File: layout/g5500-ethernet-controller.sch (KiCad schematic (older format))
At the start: 71 parts, among them IC1 MAX-M8Q, J1 CONN_01x03, J10 CONN_01x03, J11 CONN_01x02, J2 CONN_01x03, J3 MICROUSB, J4 CONN_01x02, J5 CONN_01x03, J6 CONN_01x03, J7 CONN_01x02, J8 CONN_01x02, J9 CONN_01x03, K1 G5LE-1, K2 G5LE-1, K3 G5LE-1, K4 G5LE-1, P1 COAX, Q1 BC817W, Q2 BC817W, Q3 BC817W, Q4 BC817W, U1 NUCLEO144-F429ZI, U2 LD3985G33R_TSOT23

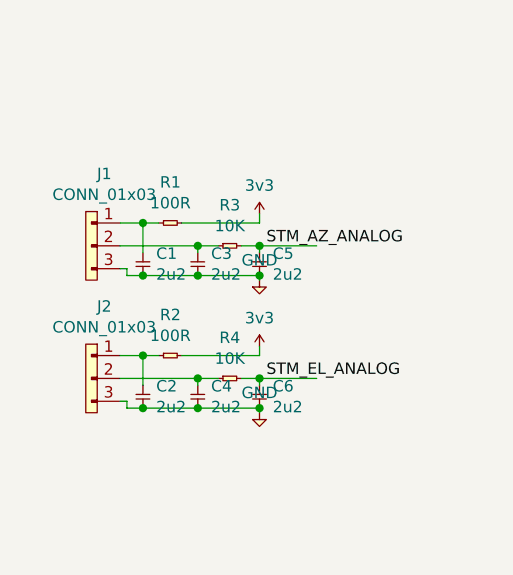
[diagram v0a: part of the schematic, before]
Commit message: layout: Finish and send off v1.
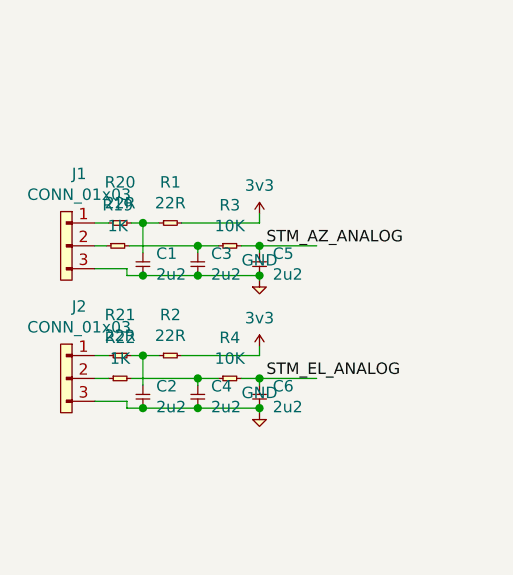
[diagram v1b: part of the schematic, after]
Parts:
- added R19, R22: 1K, agg:0603, symbol agg-kicad:R
- added R20, R21: 22R, agg:0603, symbol agg-kicad:R
- C13: footprint Capacitor_SMD:C_0603_1608Metric -> agg:0603
- R1, R2: value 100R -> 22R
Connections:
- wire segments 263 -> 267
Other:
- moved on the sheet: J1, J2
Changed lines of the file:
@@
 L agg-kicad:CONN_01x03 J2
 U 1 1 5A89F92A
-P 1680 7890
-F 0 "J2" H 1711 8105 50  0000 C CNN
-F 1 "CONN_01x03" H 1711 8014 50  0000 C CNN
-F 2 "Connector_Molex:Molex_KK-254_AE-6410-03A_1x03_P2.54mm_Vertical" H 1680 7890 50  0001 C CNN
-F 3 "" H 1680 7890 50  0001 C CNN
-	1    1680 7890
+P 1570 7890
+F 0 "J2" H 1601 8105 50  0000 C CNN
+F 1 "CONN_01x03" H 1601 8014 50  0000 C CNN
+F 2 "Connector_Molex:Molex_KK-254_AE-6410-03A_1x03_P2.54mm_Vertical" H 1570 7890 50  0001 C CNN
+F 3 "" H 1570 7890 50  0001 C CNN
+	1    1570 7890
 	1    0    0    -1
 $EndComp
@@
 P 1950 7890
 F 0 "R2" H 2000 8068 50  0000 C CNN
-F 1 "100R" H 2000 7977 50  0000 C CNN
+F 1 "22R" H 2000 7977 50  0000 C CNN
 F 2 "agg:0603" H 1950 7890 50  0001 C CNN
 F 3 "" H 1950 7890 50  0001 C CNN
@@
 Wire Wire Line
 	1880 7890 1880 8020
-Connection ~ 1880 7890
-Wire Wire Line
-	1880 7890 1780 7890
 Wire Wire Line
 	1810 8090 1810 8120
@@
 Connection ~ 2120 8120
 Wire Wire Line
-	1780 7990 2120 7990
-Wire Wire Line
 	2120 7990 2120 8020
 Wire Wire Line
 	2120 7990 2210 7990
-Connection ~ 2120 7990
 Wire Wire Line
 	2310 7990 2390 7990
@@
 L agg-kicad:CONN_01x03 J1
 U 1 1 5A8FB849
-P 1680 7310
-F 0 "J1" H 1711 7525 50  0000 C CNN
-F 1 "CONN_01x03" H 1711 7434 50  0000 C CNN
-F 2 "Connector_Molex:Molex_KK-254_AE-6410-03A_1x03_P2.54mm_Vertical" H 1680 7310 50  0001 C CNN
-F 3 "" H 1680 7310 50  0001 C CNN
-	1    1680 7310
+P 1570 7310
+F 0 "J1" H 1601 7525 50  0000 C CNN
+F 1 "CONN_01x03" H 1601 7434 50  0000 C CNN
+F 2 "Connector_Molex:Molex_KK-254_AE-6410-03A_1x03_P2.54mm_Vertical" H 1570 7310 50  0001 C CNN
+F 3 "" H 1570 7310 50  0001 C CNN
+	1    1570 7310
 	1    0    0    -1
 $EndComp
@@
 P 1950 7310
 F 0 "R1" H 2000 7488 50  0000 C CNN
-F 1 "100R" H 2000 7397 50  0000 C CNN
+F 1 "22R" H 2000 7397 50  0000 C CNN
 F 2 "agg:0603" H 1950 7310 50  0001 C CNN
 F 3 "" H 1950 7310 50  0001 C CNN
@@
 Wire Wire Line
 	1880 7310 1880 7440
-Connection ~ 1880 7310
-Wire Wire Line
-	1880 7310 1780 7310
 Wire Wire Line
 	1810 7510 1810 7540
@@
 Connection ~ 2120 7540
 Wire Wire Line
-	1780 7410 2120 7410
-Wire Wire Line
 	2120 7410 2120 7440
 Wire Wire Line
 	2120 7410 2210 7410
-Connection ~ 2120 7410
 Wire Wire Line
 	2310 7410 2390 7410
@@
 F 0 "C13" V 1844 4338 50  0000 L CNN
 F 1 "2u2" V 1935 4338 50  0000 L CNN
-F 2 "Capacitor_SMD:C_0603_1608Metric" H 1840 4280 50  0001 C CNN
+F 2 "agg:0603" H 1840 4280 50  0001 C CNN
 F 3 "" H 1840 4280 50  0001 C CNN
 	1    1840 4280
@@
 Connection ~ 1840 4250
 Wire Wire Line
-	1780 7510 1810 7510
-Wire Wire Line
-	1780 8090 1810 8090
+	1670 7510 1810 7510
+Wire Wire Line
+	1670 8090 1810 8090
 $Comp
 L agg-kicad:CONN_01x02 J7
@@
 Wire Wire Line
 	11410 2940 11410 2930
+$Comp
+L agg-kicad:R R21
+U 1 1 5AC4E62C
+P 1730 7890
+F 0 "R21" H 1780 8068 50  0000 C CNN
+F 1 "22R" H 1780 7977 50  0000 C CNN
+F 2 "agg:0603" H 1730 7890 50  0001 C CNN
+F 3 "" H 1730 7890 50  0001 C CNN
+	1    1730 7890
+	1    0    0    -1
+$EndComp
+Wire Wire Line
+	1880 7890 1830 7890
+Connection ~ 1880 7890
+Wire Wire Line
+	1730 7890 1670 7890
+$Comp
+L agg-kicad:R R22
+U 1 1 5AC9E76C
+P 1730 7990
+F 0 "R22" H 1780 8168 50  0000 C CNN
+F 1 "1K" H 1780 8077 50  0000 C CNN
+F 2 "agg:0603" H 1730 7990 50  0001 C CNN
+F 3 "" H 1730 7990 50  0001 C CNN
+	1    1730 7990
+	1    0    0    -1
+$EndComp
+Wire Wire Line
+	1830 7990 2120 7990
+Connection ~ 2120 7990
+Wire Wire Line
+	1730 7990 1670 7990
+$Comp
+L agg-kicad:R R20
+U 1 1 5AD197A9
+P 1730 7310
+F 0 "R20" H 1780 7488 50  0000 C CNN
+F 1 "22R" H 1780 7397 50  0000 C CNN
+F 2 "agg:0603" H 1730 7310 50  0001 C CNN
+F 3 "" H 1730 7310 50  0001 C CNN
+	1    1730 7310
+	1    0    0    -1
+$EndComp
+Wire Wire Line
+	1830 7310 1880 7310
+Connection ~ 1880 7310
+Wire Wire Line
+	1730 7310 1670 7310
+$Comp
+L agg-kicad:R R19
+U 1 1 5AD43024
+P 1720 7410
+F 0 "R19" H 1770 7588 50  0000 C CNN
+F 1 "1K" H 1770 7497 50  0000 C CNN
+F 2 "agg:0603" H 1720 7410 50  0001 C CNN
+F 3 "" H 1720 7410 50  0001 C CNN
+	1    1720 7410
+	1    0    0    -1
+$EndComp
+Wire Wire Line
+	1670 7410 1720 7410
+Wire Wire Line
+	1820 7410 2120 7410
+Connection ~ 2120 7410
 $EndSCHEMATC
